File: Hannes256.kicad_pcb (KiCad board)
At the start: 2 copper layers, 33.8 x 62.7 mm, 20 parts, among them J1 TED_SOCKET, J2 RAM_SELECTOR, J3 CONN_CS, U1 MOS_7360_TED, U2 74LS257, U3 74LS257, U4 XX4256, U5 XX4256, U6 GAL20V8, U7 74HCT74, U8 74HCT74

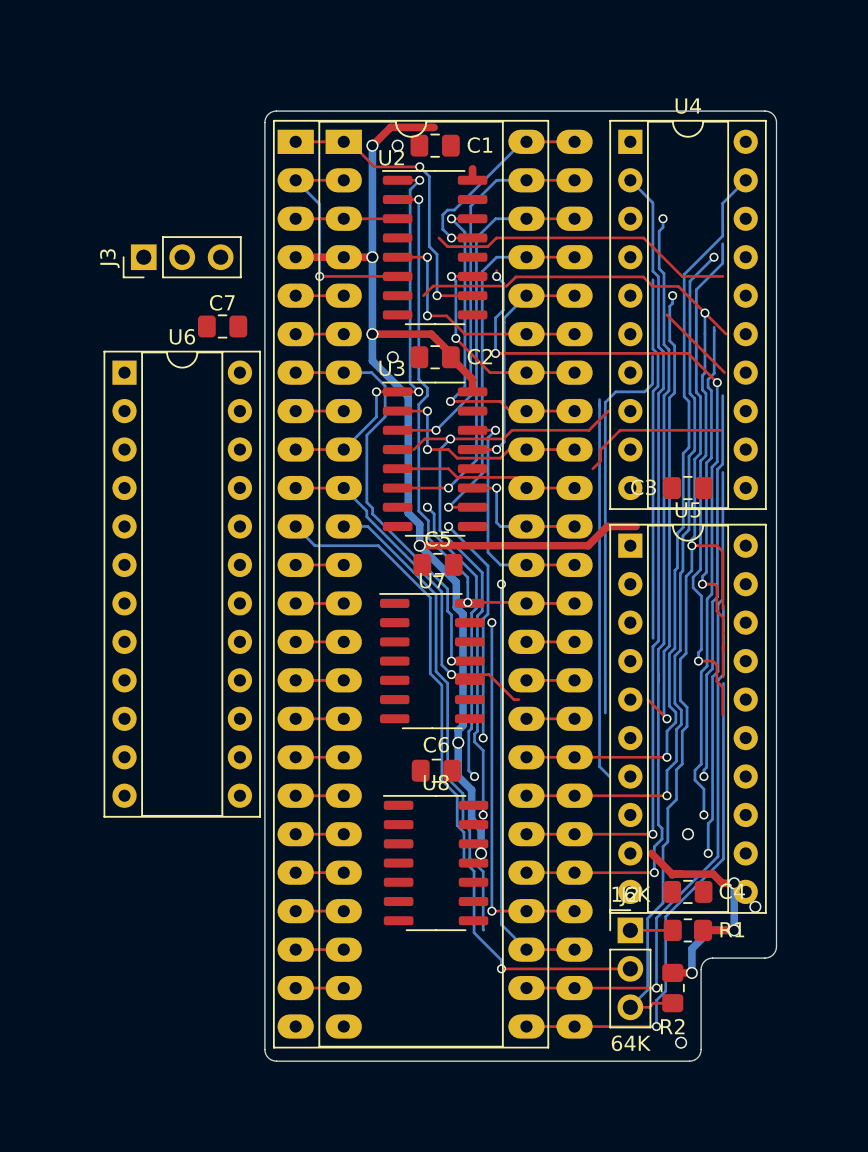
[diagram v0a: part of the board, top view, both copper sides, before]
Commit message: Routing in progress
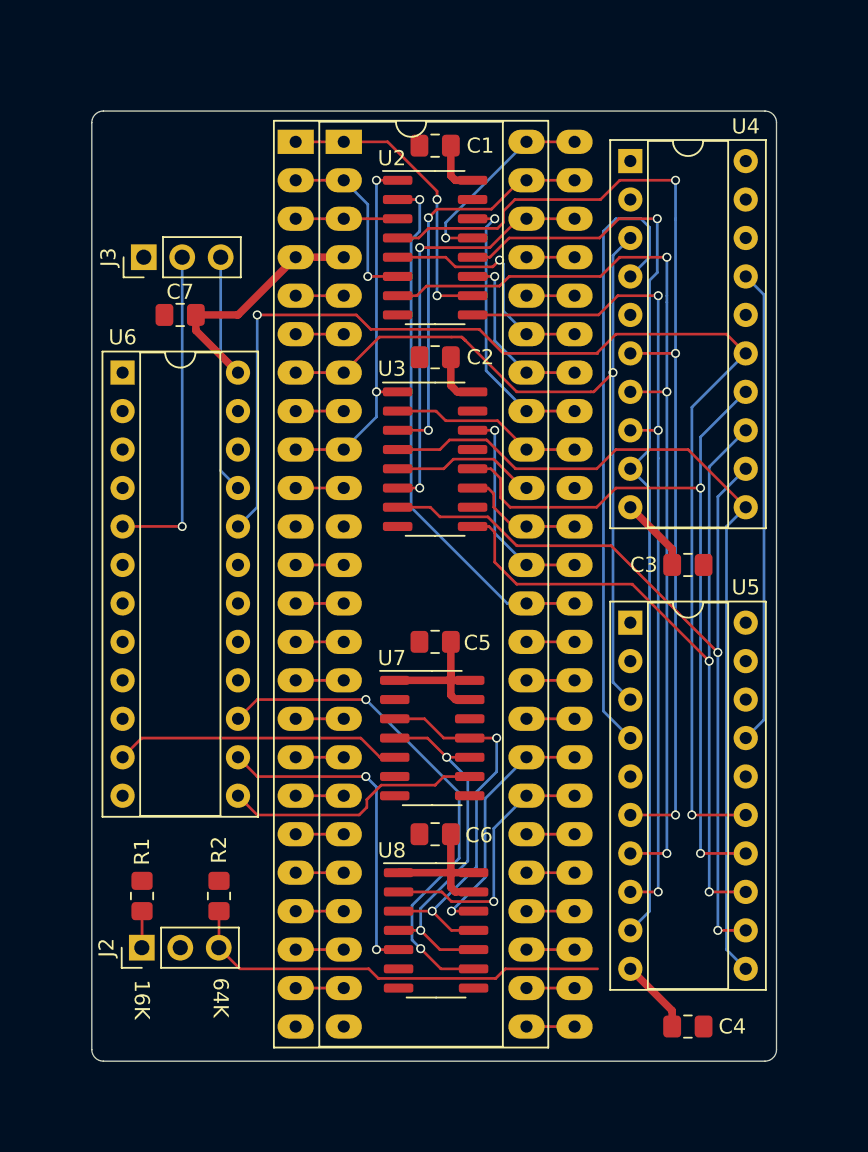
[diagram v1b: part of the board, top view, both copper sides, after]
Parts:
- moved R1 36.1 mm to (111.8, 125.7), turned to 270 degrees
- moved J2 32.3 mm to (111.8, 129.2), turned to 90 degrees
- moved R2 30.6 mm to (116.9, 125.7)
- moved C4 8.89 mm to (147.8, 134.4)
- moved C5 5.08 mm to (131.1, 109.0), turned to 180 degrees
- moved C3 5.08 mm to (147.8, 103.9)
- moved U5 5.08 mm to (144.0, 107.7)
- moved U7 5.08 mm to (130.9, 115.3)
- moved U8 4.44 mm to (131.2, 128.0)
- moved C6 4.19 mm to (131.1, 121.7), turned to 180 degrees
- moved C7 2.91 mm to (114.3, 87.4)
- moved U4 1.27 mm to (144.0, 77.2)
- moved U6 0.13 mm to (110.5, 91.2)
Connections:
- net Net-(U6-Pad11) renamed /~RAS~/~CAS~ Generation/p0
- net Net-(U6-Pad13) renamed /~RAS~/~CAS~ Generation/p1
- net Net-(U6-Pad14) renamed /~RAS~/~CAS~ Generation/p6
- net Net-(U6-Pad15) renamed /~RAS~/~CAS~ Generation/p7
- C2 pad 1: VCC -> +5V
- C7 pad 1: VCC -> +5V
- J1 pad 4: VCC -> +5V
- R1 pad 1: VCC -> +5V
- R2 pad 1: VCC -> +5V
- U1 pad 4: VCC -> +5V
- U2 pad 16: VCC -> +5V
- U3 pad 16: VCC -> +5V
- U6 pad 6: a0 -> a12
- U6 pad 7: a1 -> a13
- U6 pad 8: a2 -> a14
- U6 pad 9: a3 -> a15
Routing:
- net VCC: track 102.8 -> 0.00 mm, vias 9 -> 0
- net m8: track 0.00 -> 84.4 mm, vias 0 -> 2
- net m0: track 0.00 -> 68.3 mm, vias 0 -> 3
- net m1: track 0.00 -> 63.0 mm, vias 0 -> 3
- net m3: track 0.00 -> 62.0 mm, vias 0 -> 1
- net m5: track 0.00 -> 58.2 mm, vias 0 -> 2
- net m4: track 0.00 -> 57.7 mm
- net m2: track 0.00 -> 55.8 mm, vias 0 -> 3
- net m6: track 0.00 -> 54.4 mm, vias 0 -> 2
- net +5V: track 0.00 -> 53.7 mm, vias 1 -> 0
- net m7: track 0.00 -> 52.1 mm, vias 0 -> 2
- net /64K RAM Expansion/m1: track 50.7 -> 0.00 mm, vias 2 -> 0
- net /64K RAM Expansion/m3: track 50.7 -> 0.00 mm, vias 4 -> 0
- net d4: track 53.0 -> 3.18 mm, vias 2 -> 0
- net d5: track 52.9 -> 3.18 mm, vias 1 -> 0
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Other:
- board size 33.8 x 62.7 mm -> 45.2 x 62.7 mm

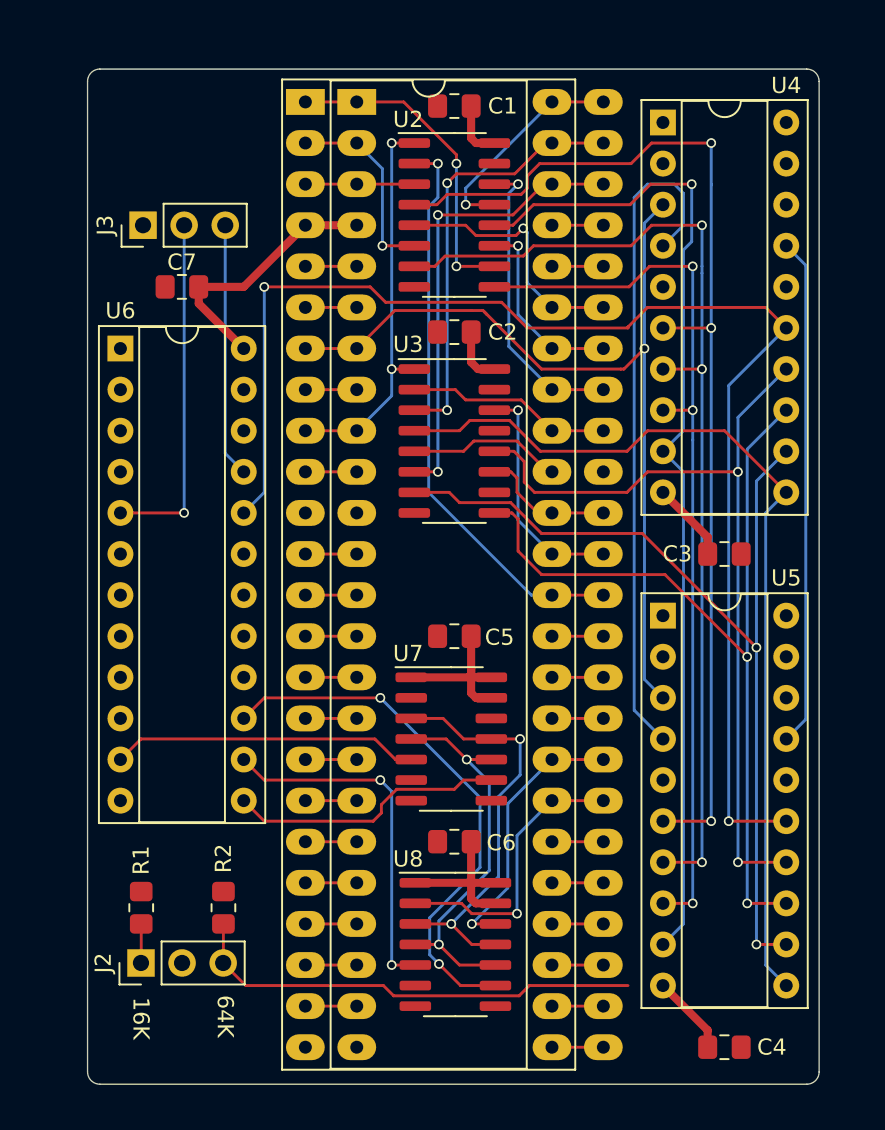
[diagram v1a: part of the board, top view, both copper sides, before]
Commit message: Routing in progress
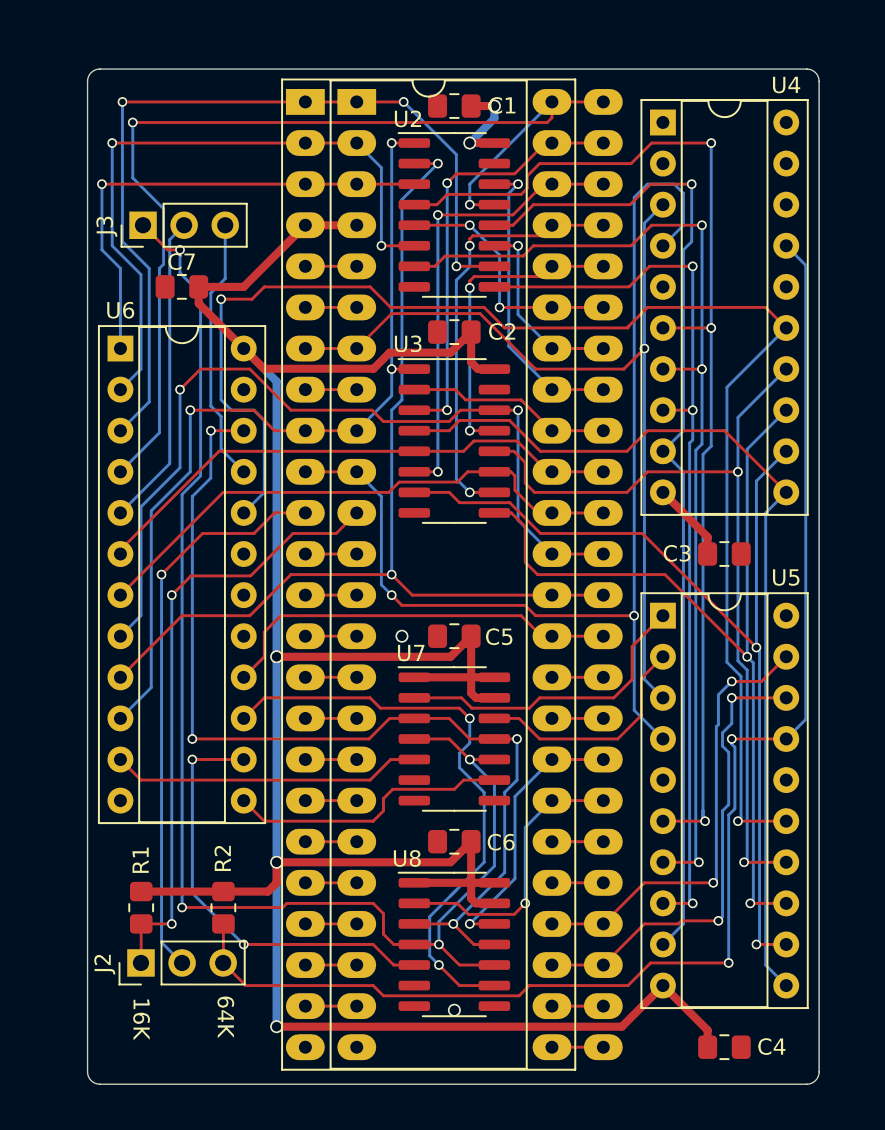
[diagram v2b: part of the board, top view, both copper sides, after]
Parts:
- moved U7 0.19 mm to (131.1, 115.3)
- moved U8 0.06 mm to (131.1, 128.0)
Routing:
- net +5V: track 53.7 -> 173.9 mm, vias 0 -> 5
- net ~RESET: track 24.2 -> 85.4 mm, vias 2 -> 4
- net a3: track 13.5 -> 63.6 mm, vias 1 -> 2
- net a14: track 14.4 -> 52.7 mm, vias 1 -> 2
- net /~cas_16k: track 2.42 -> 38.2 mm, vias 0 -> 2
- net /~RAS~/~CAS~ Generation/~cs_ram: track 25.9 -> 61.2 mm, vias 2 -> 4
- net /~cas: track 0.00 -> 35.0 mm, vias 0 -> 1
- net a2: track 19.9 -> 53.0 mm, vias 2 -> 3
- net a1: track 12.2 -> 40.6 mm, vias 1 -> 2
- net MUX: track 24.6 -> 53.1 mm, vias 2 -> 3
- net a13: track 8.31 -> 34.6 mm
- net d2: track 3.18 -> 29.2 mm, vias 0 -> 2
- net a15: track 35.4 -> 61.0 mm, vias 1 -> 2
- net ~RAS: track 44.8 -> 69.7 mm, vias 0 -> 2
- net d3: track 3.18 -> 27.9 mm, vias 0 -> 2
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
